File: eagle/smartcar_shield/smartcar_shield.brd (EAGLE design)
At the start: 49.5 x 53.2 mm, 18 parts, among them IC1 L293D, J1 ARDUINO_R3_SHIELD

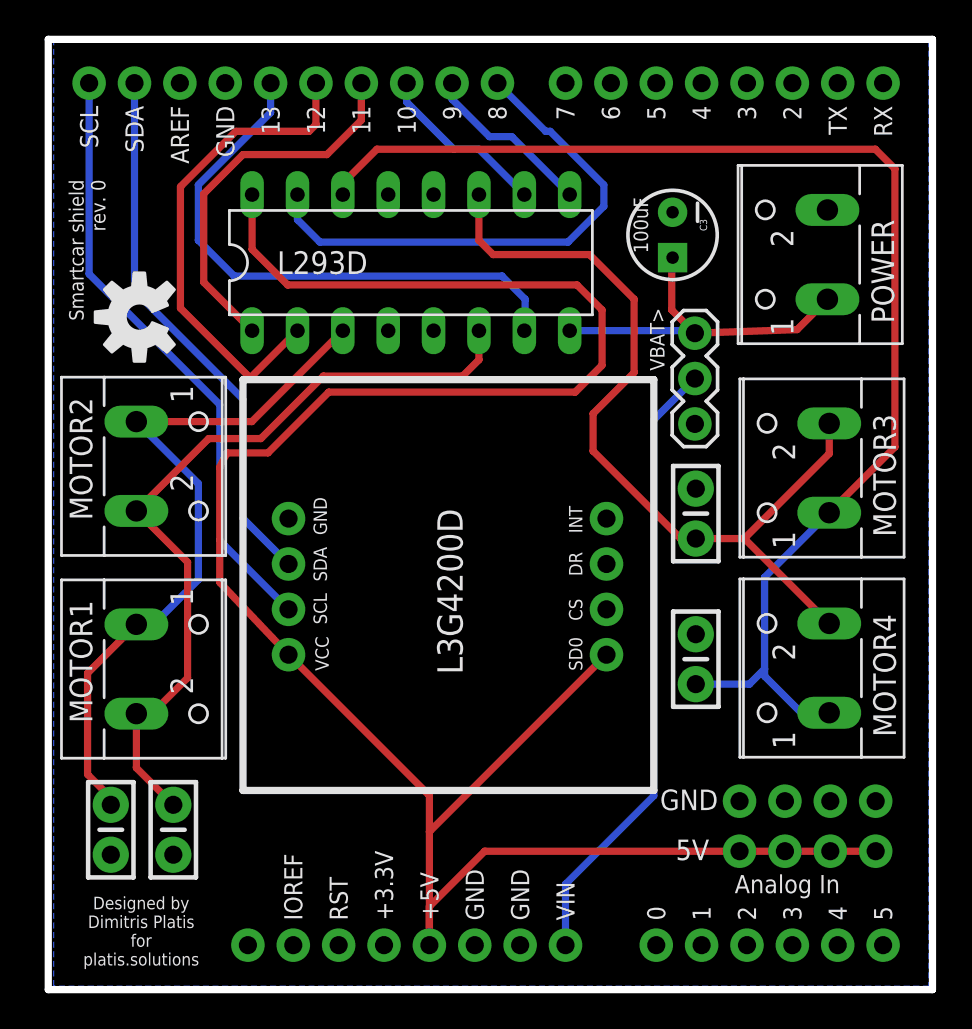
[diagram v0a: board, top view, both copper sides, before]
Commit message: smartcar shield rev. 1
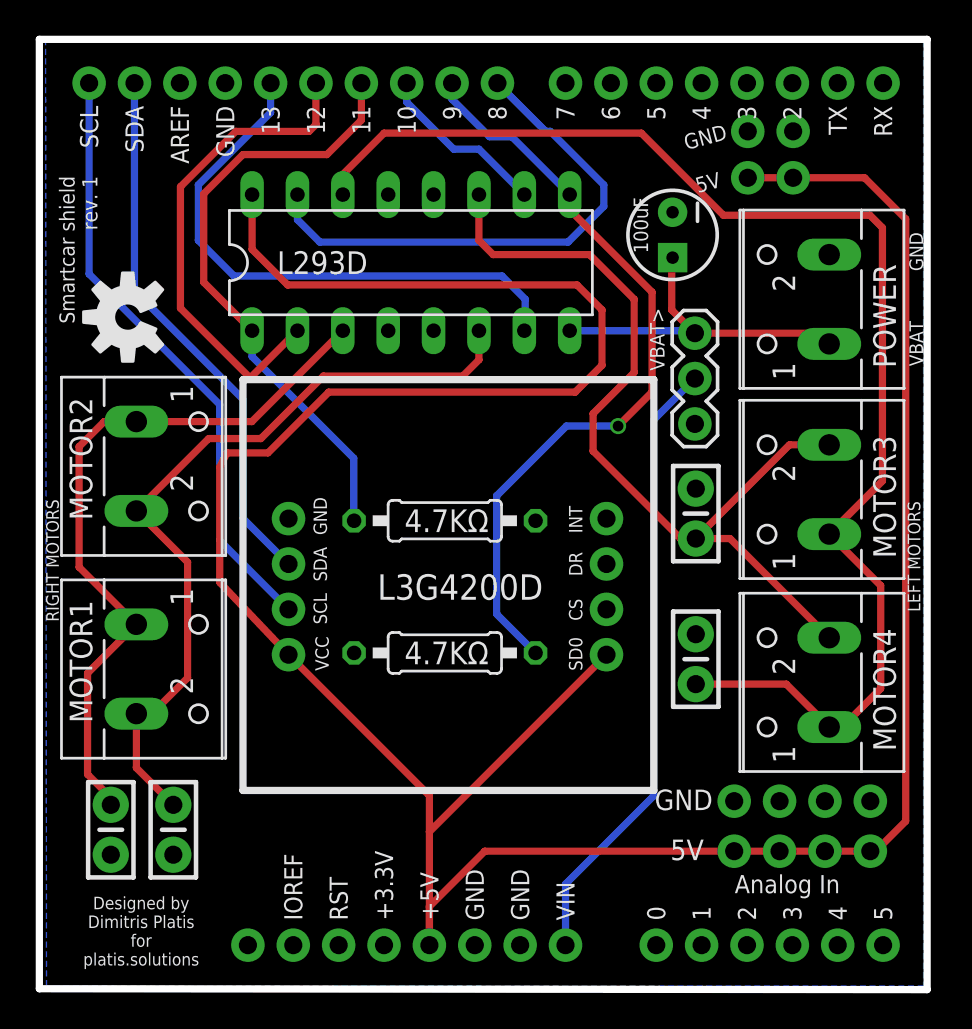
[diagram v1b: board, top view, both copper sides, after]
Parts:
- added JP8, JP9: (no value), SparkFun-Connectors:1X02_NO_SILK
- added R1, R2: 4.7KΩ, rcl:0207/10
- moved POWER 2.50 mm to (42.5, 38.7)
- moved MOTOR3 1.20 mm to (42.5, 28.1)
- moved MOTOR4 0.80 mm to (42.5, 17.2)
- moved U$1 0.65 mm to (4.45, 37.7)
- moved JP4 0.30 mm to (38.4, 10.6)
- moved JP5 0.30 mm to (38.4, 7.80)
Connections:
- net +5V: now also JP8.1, JP8.2
- net ENABLE1: now also R1.1
- net ENABLE2: now also R2.2
- net GND: now also JP9.1, JP9.2, R1.2, R2.1
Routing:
- net +5V: track 125.1 -> 171.0 mm
- net ENABLE2: track 9.70 -> 43.5 mm, vias 0 -> 1
- net ENABLE1: track 21.4 -> 34.4 mm
- net MOTORB-OUT1: track 72.9 -> 75.0 mm
- net MOTORB-OUT2: track 47.7 -> 49.3 mm
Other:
- board size 49.5 x 53.2 mm -> 49.7 x 53.2 mm
- board text added: "Find documentation at http://plat.is/smartcar"
- board text added: "GND 5V"
- board text added: "LEFT MOTORS"
- board text added: "RIGHT MOTORS"
- board text added: "Smartcar shield rev. 1"
- board text added: "VBAT"
- board text removed: "Smartcar shield rev. 0"
